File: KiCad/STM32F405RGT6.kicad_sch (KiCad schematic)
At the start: 48 parts, among them IC1 FT232RQ-REEL, J1 USB_C_Receptacle_USB2.0, J2 USB_C_Receptacle_USB2.0, SW1 SW_SPST, U1 STM32F405RGTx, U2 AT24CS64-SSHM, Y1 25MHz

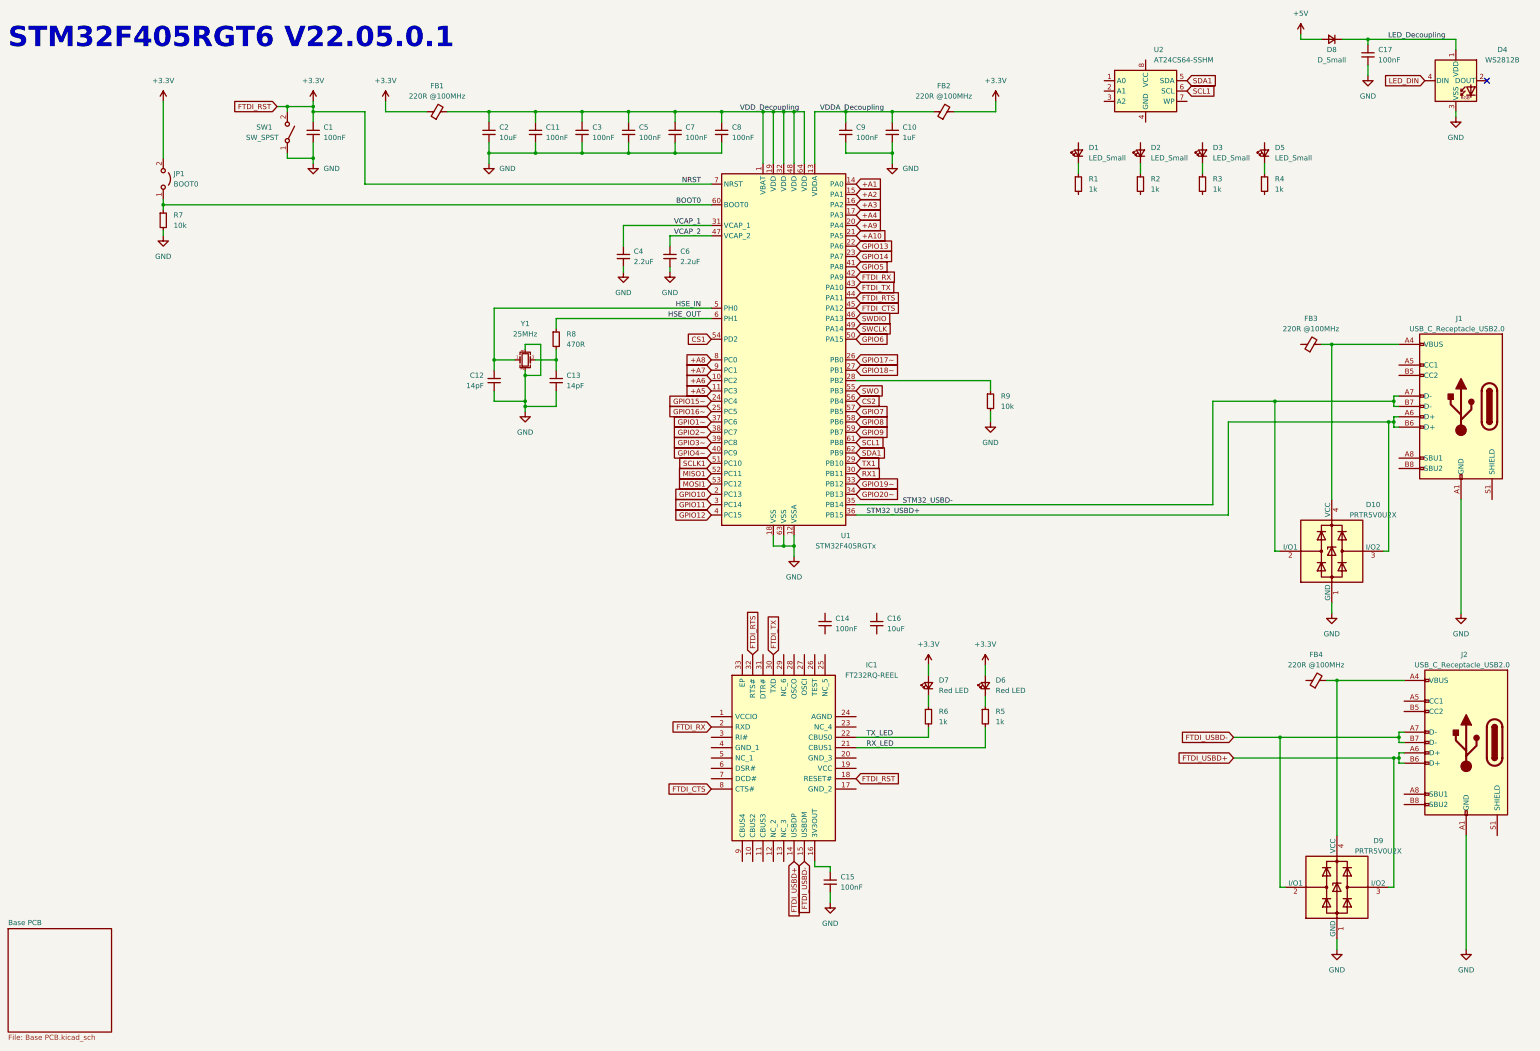
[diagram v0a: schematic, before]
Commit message: Updated PCB and Schematic
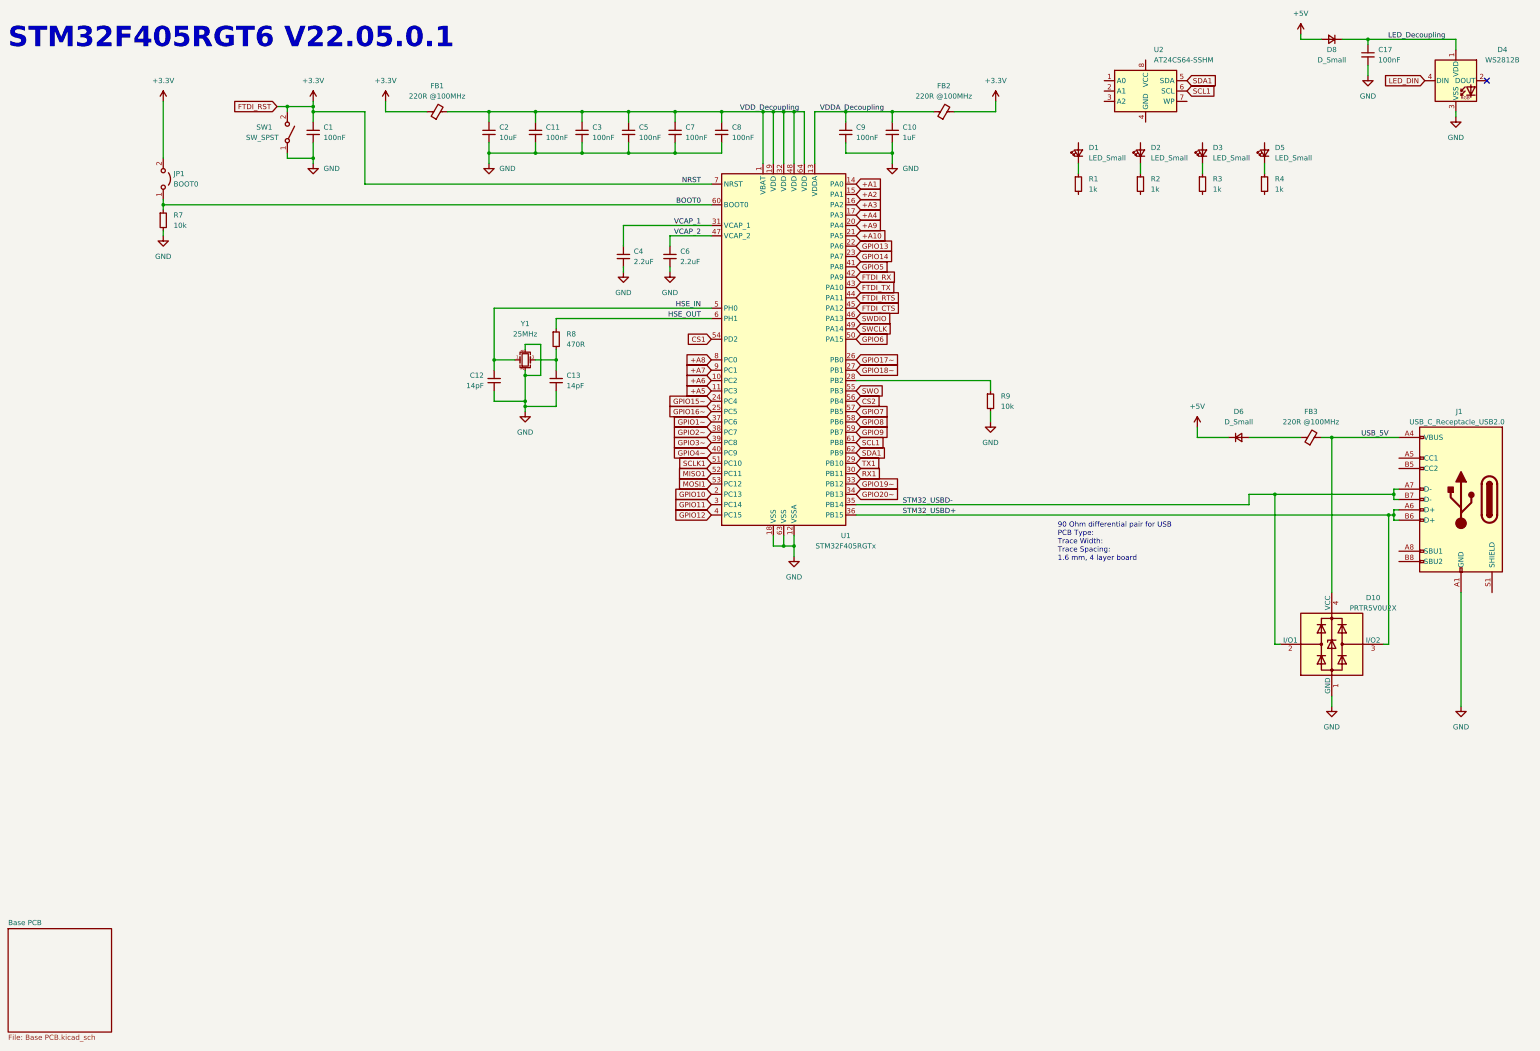
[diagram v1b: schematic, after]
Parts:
- removed C14, C15: 100nF, Capacitor_SMD:C_0603_1608Metric, symbol Device:C_Small
- removed C16: 10uF, Capacitor_SMD:C_0603_1608Metric, symbol Device:C_Small
- removed D6, D7: Red LED, LED_SMD:LED_0603_1608Metric, symbol Device:LED_Small
- removed D9: PRTR5V0U2X, Package_TO_SOT_SMD:SOT-143, symbol Power_Protection:PRTR5V0U2X
- removed FB4: 220R @100MHz, Inductor_SMD:L_0603_1608Metric, symbol Device:FerriteBead_Small
- removed IC1: FT232RQ-REEL, Package_DFN_QFN:QFN-32-1EP_5x5mm_P0.5mm_EP3.3x3.3mm_ThermalVias, symbol FT232RQ-REEL:FT232RQ-REEL
- removed J2: USB_C_Receptacle_USB2.0, Connector_USB:USB_C_Receptacle_HRO_TYPE-C-31-M-12, symbol Connector:USB_C_Receptacle_USB2.0
- removed R5, R6: 1k, Resistor_SMD:R_0603_1608Metric, symbol Device:R_Small
- added D6: D_Small, symbol Device:D_Small
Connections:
- net +5V: now also D6.1 (K)
- net USB_5V: now reaches D10.4 (VCC), FB3.2, J1.A4 (VBUS), J1.A9 (VBUS), J1.B4 (VBUS), J1.B9 (VBUS)
- net at FB3.1: now also D6.2 (A)
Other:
- note added: "90 Ohm differential pair for USB PCB Type: Trace Width: Trace Spacing: 1.6 mm, 4 layer board"
- moved on the sheet: D10, FB3, J1
